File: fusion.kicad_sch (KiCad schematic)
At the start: 67 parts, among them J1 Conn_01x04_Female, J2 USB_C_Receptacle_USB2.0, J3 Conn_01x22, J4 Conn_01x22, K1 KEY, K10 KEY, K11 KEY, K12 KEY, K13 KEY, K14 KEY, K15 KEY, K16 KEY, K17 KEY, K18 KEY, K19 KEY, K2 KEY, K20 KEY, K21 KEY, K22 KEY, K23 KEY, K24 KEY, K25 KEY, K26 KEY, K27 KEY, K28 KEY, K29 KEY, K3 KEY, K30 KEY, K31 KEY, K32 KEY, K33 KEY, K34 KEY, K35 KEY, K36 KEY, K37 KEY, K38 KEY, K4 KEY, K5 KEY, K6 KEY, K7 KEY, K8 KEY, K9 KEY, SW1 SW_Push, U1 Holyiot_18010, U2 MT25QL128ABA1ESE, U3 BQ24075, U4 XC6220B331MR, U5 LN4913

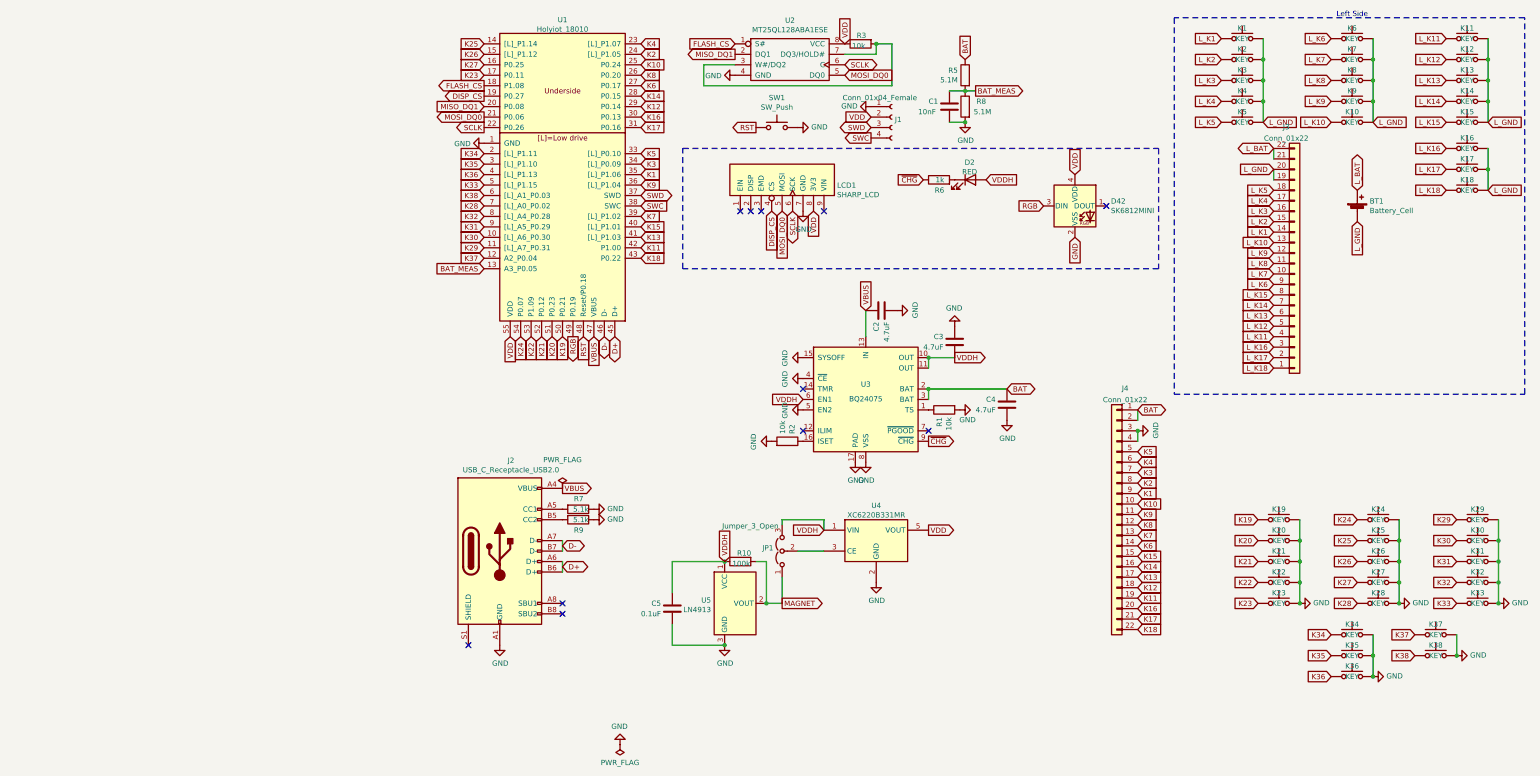
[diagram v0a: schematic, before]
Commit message: bug
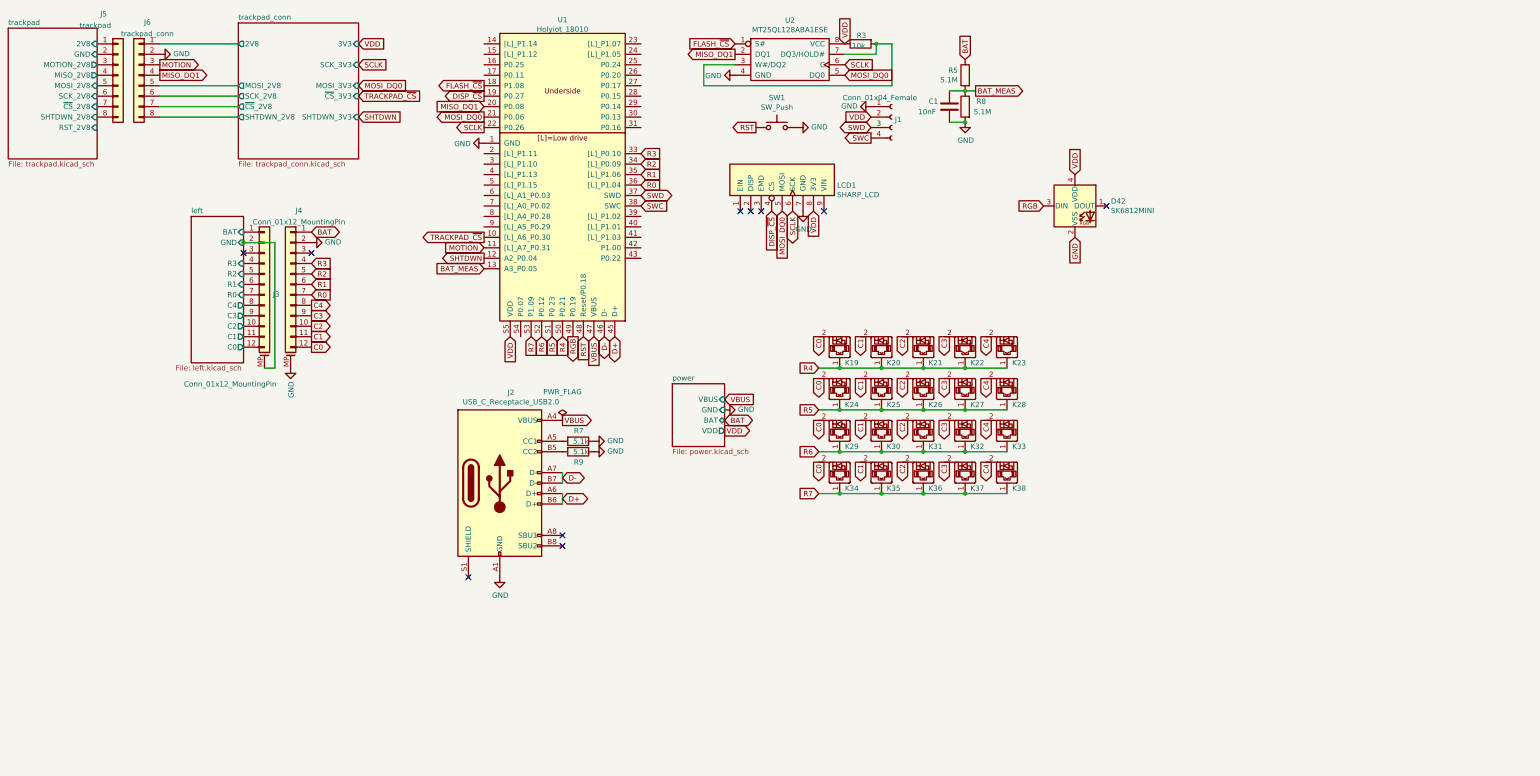
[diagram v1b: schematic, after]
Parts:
- removed BT1: Battery_Cell, Connector_JST:JST_PH_S2B-PH-K_1x02_P2.00mm_Horizontal, symbol Device:Battery_Cell
- removed C2, C3, C4: 4.7uF, Capacitor_SMD:C_0603_1608Metric, symbol Device:C
- removed C5: 0.1uF, Capacitor_SMD:C_0603_1608Metric, symbol Device:C
- removed D2: RED, LED_SMD:LED_0805_2012Metric, symbol Device:LED
- removed J3, J4: Conn_01x22, Connector_FFC-FPC:Hirose_FH12-22S-0.5SH_1x22-1MP_P0.50mm_Horizontal, symbol Connector_Generic:Conn_01x22
- removed JP1: Jumper_3_Open, Jumper:SolderJumper-3_P2.0mm_Open_TrianglePad1.0x1.5mm_NumberLabels, symbol Jumper:Jumper_3_Open
- removed K1, K10, K11, K15, K37, K38, K5, K6: KEY, keeb-libs:pg1232-shorter-right, symbol Switch:SW_Push
- removed K12, K13, K16, K17, K18, K2, K21, K22, K26, K27, K3, K31, K32, K34, K35, K36, K7, K8: KEY, keeb-libs:pg1232-short, symbol Switch:SW_Push
- removed K14, K4, K9: KEY, keeb-libs:pg1232-short-left, symbol Switch:SW_Push
- removed K19, K23, K24, K28, K29, K33: KEY, keeb-libs:pg1232-shorter-left, symbol Switch:SW_Push
- removed K20, K25, K30: KEY, keeb-libs:pg1232-short-right, symbol Switch:SW_Push
- removed R1, R2: 10k, Resistor_SMD:R_0603_1608Metric, symbol Device:R
- removed R10: 100k, Resistor_SMD:R_0603_1608Metric, symbol Device:R
- removed R6: 1k, Resistor_SMD:R_0603_1608Metric, symbol Device:R
- removed U3: BQ24075, Package_DFN_QFN:VQFN-16-1EP_3x3mm_P0.5mm_EP1.68x1.68mm_ThermalVias, symbol Battery_Management:BQ24075
- removed U4: XC6220B331MR, Package_TO_SOT_SMD:SOT-23-5, symbol Regulator_Linear:XC6220B331MR
- removed U5: LN4913, Package_TO_SOT_SMD:SOT-23, symbol Sensor_Magnetic:A1101ELHL
- added J3, J4: Conn_01x12_MountingPin, Connector_FFC-FPC:Hirose_FH12-12S-0.5SH_1x12-1MP_P0.50mm_Horizontal, symbol Connector_Generic_MountingPin:Conn_01x12_MountingPin
- added J5: trackpad, fusion:trackpad, symbol Connector_Generic:Conn_01x08
- added J6: trackpad_conn, fusion:trackpad_conn, symbol Connector_Generic:Conn_01x08
- added K19, K23, K24, K28, K29, K33: diode-choc, pg1232:pg1232-DSSL, symbol diode-choc:diode-choc
- added K20, K25, K30, K37, K38: diode-choc, pg1232:pg1232-DSSR, symbol diode-choc:diode-choc
- added K21, K22, K26, K27, K31, K32, K34, K35, K36: diode-choc, pg1232:pg1232-DSS, symbol diode-choc:diode-choc
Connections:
- net BAT: now also J4.1 (Pin_1)
- net GND: now also J4.2 (Pin_2), J4.MP (MountPin), J6.2 (Pin_2)
- net MISO_DQ1: now also J6.4 (Pin_4)
- net DISP_CS renamed DISP_~{CS}
- net FLASH_CS renamed FLASH_~{CS}
- net K1 renamed R1
- net R1: now also J4.6 (Pin_6)
- net K10: no longer names the net of U1.25 (P0.24)
- net K11: no longer names the net of U1.42 (P1.00)
- net K12: no longer names the net of U1.29 (P0.14)
- net K13: no longer names the net of U1.41 ([L]_P1.03)
- net K14: no longer names the net of U1.28 (P0.15)
- net K15: no longer names the net of U1.40 ([L]_P1.01)
- net K16: no longer names the net of U1.30 (P0.13)
- net K17: no longer names the net of U1.31 (P0.16)
- net K18: no longer names the net of U1.43 (P0.22)
- net K19 renamed R4
- net R4: now also K19.1, K20.1, K21.1, K22.1, K23.1
- net K2: no longer names the net of U1.24 ([L]_P1.05)
- net K20 renamed R5
- net R5: now also K24.1, K25.1, K26.1, K27.1, K28.1
- net K21 renamed R6
- net R6: now also K29.1, K30.1, K31.1, K32.1, K33.1
- net K22 renamed R7
- net R7: now also K34.1, K35.1, K36.1, K37.1, K38.1
- net K23: no longer names the net of U1.17 (P0.11)
- net K24: no longer names the net of U1.54 (P0.07)
- net K25: no longer names the net of U1.14 ([L]_P1.14)
- net K26: no longer names the net of U1.15 ([L]_P1.12)
- net K27: no longer names the net of U1.16 (P0.25)
- net K28: no longer names the net of U1.7 ([L]_A0_P0.02)
- net K29 renamed MOTION
- net MOTION: now also J6.3 (Pin_3)
- net K3 renamed R2
- net R2: now also J4.5 (Pin_5)
- net K30 renamed TRACKPAD_~{CS}
- net K31: no longer names the net of U1.9 ([L]_A5_P0.29)
- net K32: no longer names the net of U1.8 ([L]_A4_P0.28)
- net K33: no longer names the net of U1.5 ([L]_P1.15)
- net K34: no longer names the net of U1.2 ([L]_P1.11)
- net K35: no longer names the net of U1.3 ([L]_P1.10)
- net K36: no longer names the net of U1.4 ([L]_P1.13)
- net K37 renamed SHTDWN
- net K38: no longer names the net of U1.6 ([L]_A1_P0.03)
- net K4: no longer names the net of U1.23 ([L]_P1.07)
- net K5 renamed R3
- net R3: now also J4.4 (Pin_4)
- net K6: no longer names the net of U1.27 (P0.17)
- net K7: no longer names the net of U1.39 ([L]_P1.02)
- net K8: no longer names the net of U1.26 (P0.20)
- net K9 renamed R0
- net R0: now also J4.7 (Pin_7)
- new net C0: J4.12 (Pin_12), K19.2, K24.2, K29.2, K34.2
- new net C1: J4.11 (Pin_11), K20.2, K25.2, K30.2, K35.2
- new net C2: J4.10 (Pin_10), K21.2, K26.2, K31.2, K36.2
- new net C3: J4.9 (Pin_9), K22.2, K27.2, K32.2, K37.2
- new net C4: J4.8 (Pin_8), K23.2, K28.2, K33.2, K38.2
- new net left/BAT: J3.1 (Pin_1)
- new net left/C0: J3.12 (Pin_12)
- new net left/C1: J3.11 (Pin_11)
- new net left/C2: J3.10 (Pin_10)
- new net left/C3: J3.9 (Pin_9)
- new net left/C4: J3.8 (Pin_8)
- new net left/GND: J3.2 (Pin_2), J3.MP (MountPin)
- new net left/R0: J3.7 (Pin_7)
- new net left/R1: J3.6 (Pin_6)
- new net left/R2: J3.5 (Pin_5)
- new net left/R3: J3.4 (Pin_4)
- new net trackpad/2V8: J5.1 (Pin_1)
- new net trackpad/GND: J5.2 (Pin_2)
- new net trackpad/MISO_2V8: J5.4 (Pin_4)
- new net trackpad/MOSI_2V8: J5.5 (Pin_5)
- new net trackpad/MOTION_2V8: J5.3 (Pin_3)
- new net trackpad/SCK_2V8: J5.6 (Pin_6)
- new net trackpad/SHTDWN_2V8: J5.8 (Pin_8)
- new net trackpad/~{CS}_2V8: J5.7 (Pin_7)
- new net trackpad_conn/2V8: J6.1 (Pin_1)
- new net trackpad_conn/MOSI_2V8: J6.5 (Pin_5)
- new net trackpad_conn/SCK_2V8: J6.6 (Pin_6)
- new net trackpad_conn/SHTDWN_2V8: J6.8 (Pin_8)
- new net trackpad_conn/~{CS}_2V8: J6.7 (Pin_7)
- no-connect marks 11 -> 10
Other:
- added sheet left (left.kicad_sch)
- added sheet power (power.kicad_sch)
- added sheet trackpad (trackpad.kicad_sch)
- added sheet trackpad_conn (trackpad_conn.kicad_sch)
- note removed: "Left Side"
- moved on the sheet: J2, R7, R9

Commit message: trackpad
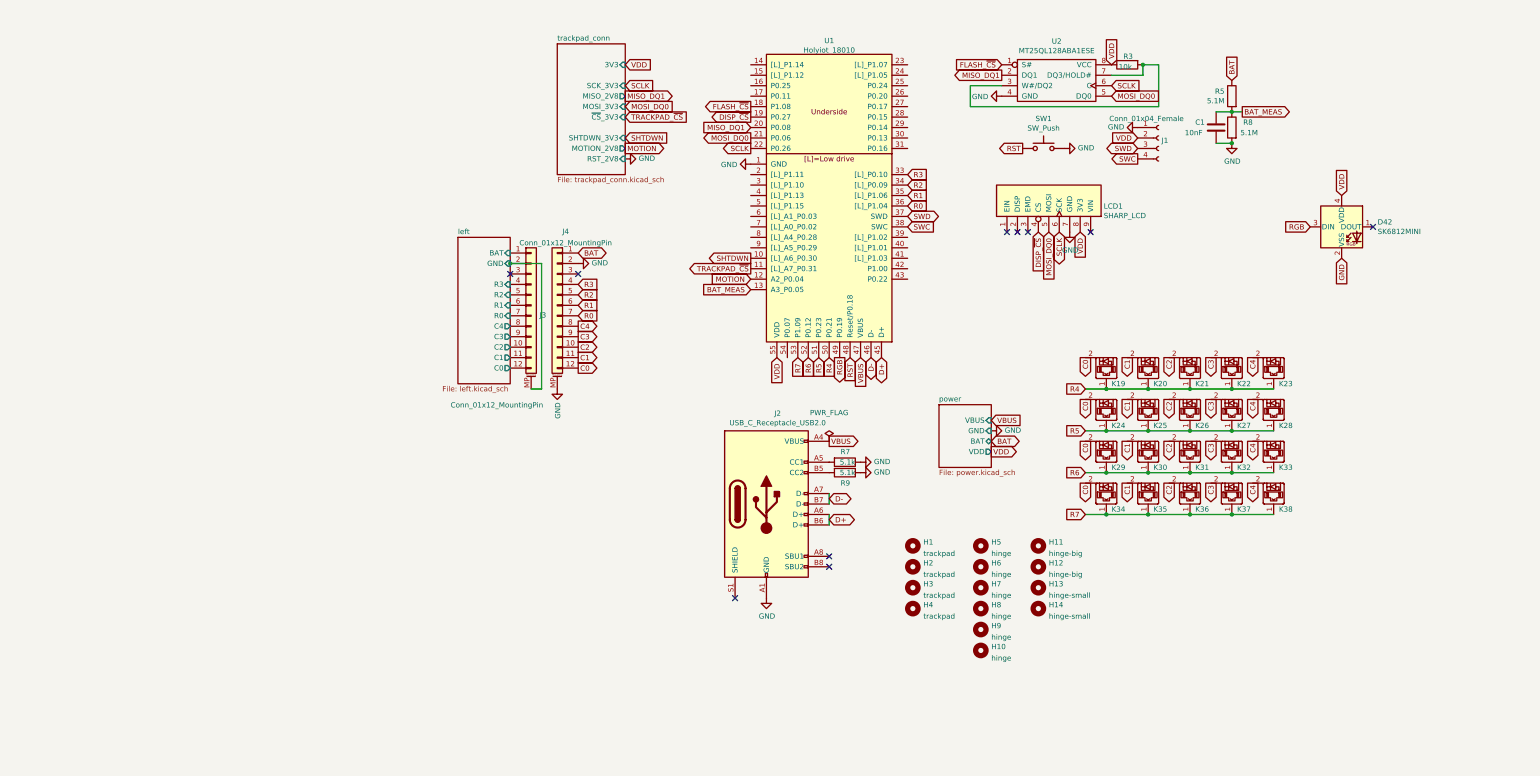
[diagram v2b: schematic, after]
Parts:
- removed J5: trackpad, fusion:trackpad, symbol Connector_Generic:Conn_01x08
- removed J6: trackpad_conn, fusion:trackpad_conn, symbol Connector_Generic:Conn_01x08
- added H1, H2, H3, H4: trackpad, fusion:trackpad, symbol Mechanical:MountingHole
- added H10, H5, H6, H7, H8, H9: hinge, fusion:hinge, symbol Mechanical:MountingHole
- added H11, H12: hinge-big, fusion:hinge-big, symbol Mechanical:MountingHole
- added H13, H14: hinge-small, fusion:hinge-small, symbol Mechanical:MountingHole
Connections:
- net MOTION: now also U1.12 (A2_P0.04); no longer U1.11 ([L]_A7_P0.31)
- net SHTDWN: now also U1.10 ([L]_A6_P0.30); no longer U1.12 (A2_P0.04)
- net TRACKPAD_~{CS}: now also U1.11 ([L]_A7_P0.31); no longer U1.10 ([L]_A6_P0.30)
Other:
- removed sheet trackpad
- sheet trackpad_conn ports: added MISO_2V8, MOTION_2V8, RST_2V8; removed 2V8, MOSI_2V8, SCK_2V8, SHTDWN_2V8, ~{CS}_2V8
- moved on the sheet: C1, D42, J1, J2, J3, J4, K19, K20, K21, K22, K23, K24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
